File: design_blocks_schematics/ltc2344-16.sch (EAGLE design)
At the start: 6 parts

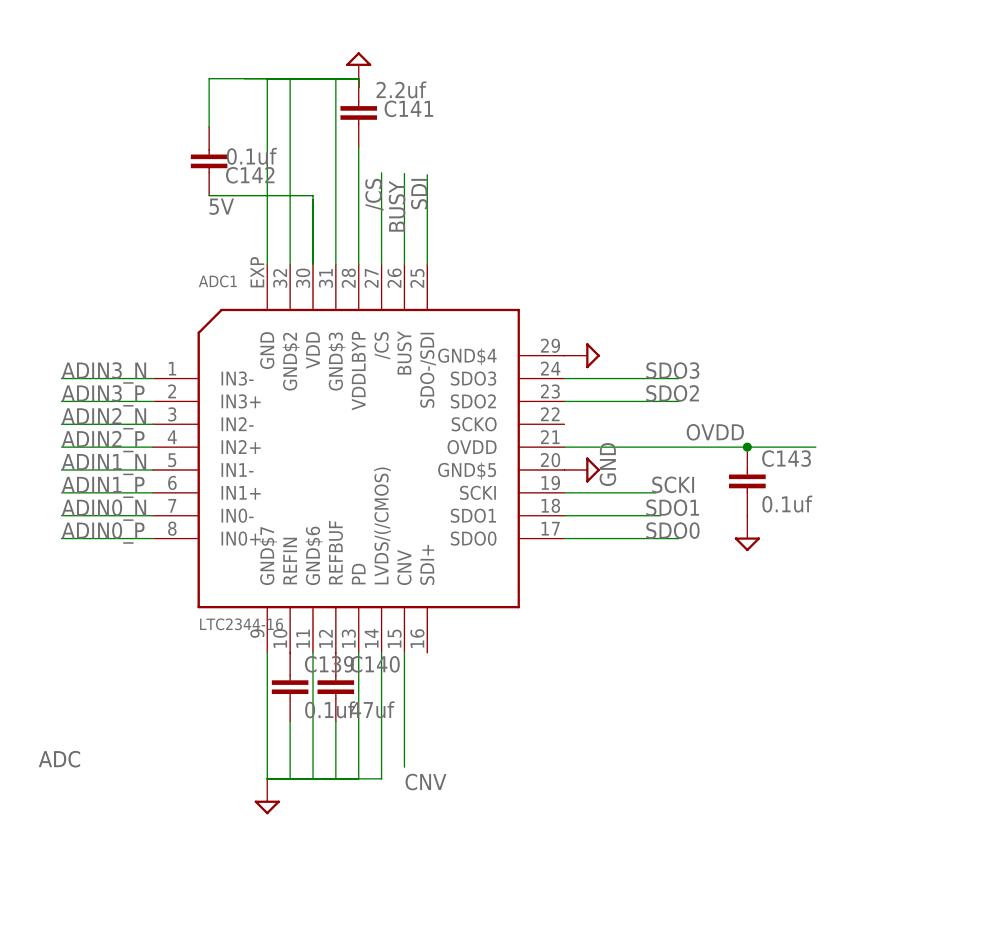
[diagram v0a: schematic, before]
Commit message: update on adc
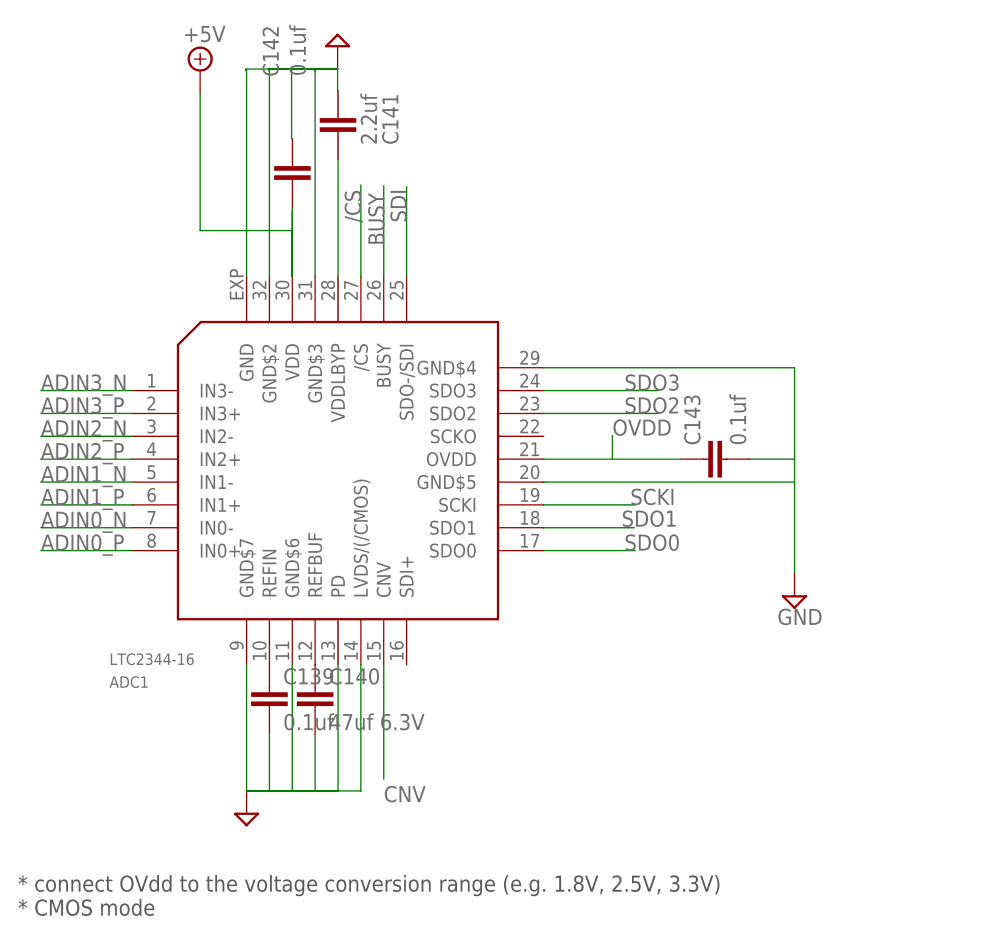
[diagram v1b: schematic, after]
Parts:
- C140: value 47uf -> 47uf 6.3V; device rcl:C-EUC1210 -> rcl:C-EUC0603
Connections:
- net 5V renamed +5V
- net OVDD renamed N$1
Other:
- note added: "* connect OVdd to the voltage conversion range (e.g. 1.8V, 2.5V, 3.3V) * CMOS mode"
- note removed: "ADC"
- moved on the sheet: ADC1, C139, C140, C141, C142, C143
